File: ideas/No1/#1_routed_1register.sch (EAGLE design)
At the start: 20 parts, among them P1-O8RIGHT TD620831A, P1-P8LEFT TD620831A, U1 SN74HC595N, U2 SN74HC595N, U3 SN74HC595N

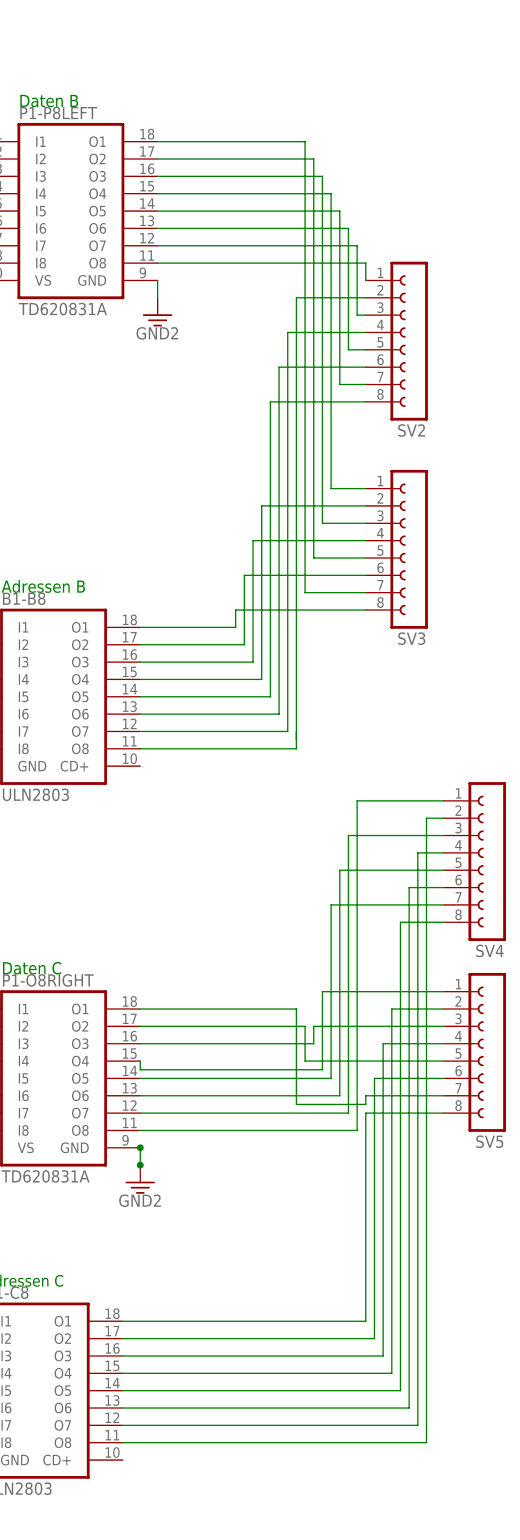
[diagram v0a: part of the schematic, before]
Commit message: 1_route_1register.sch updated
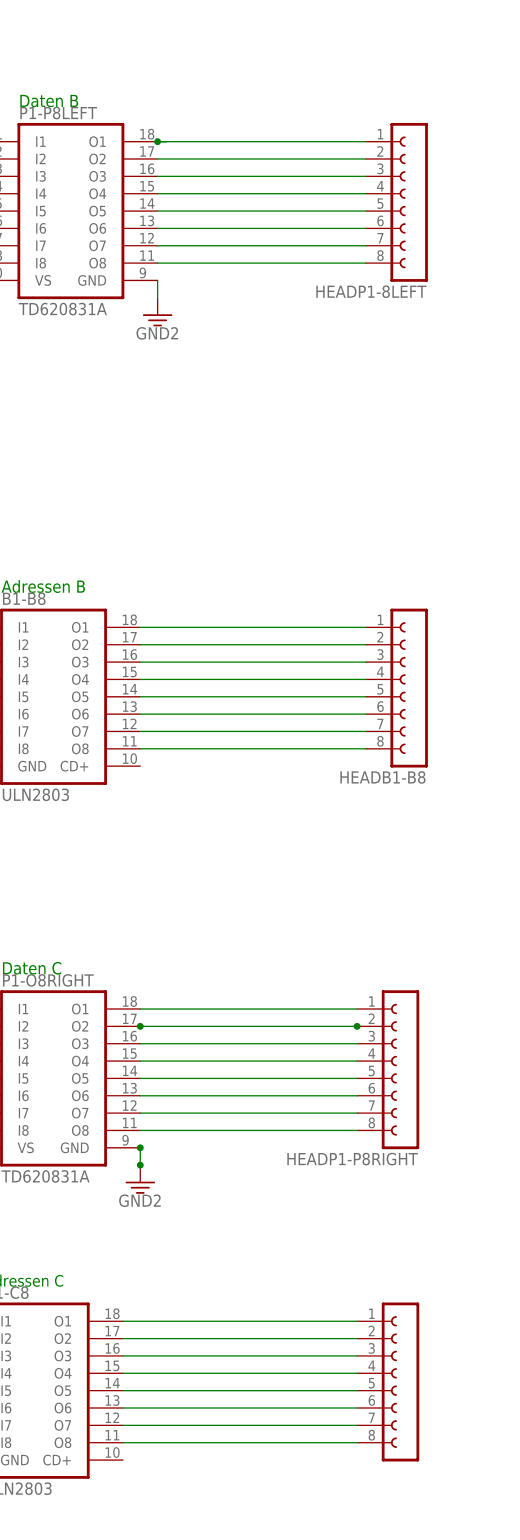
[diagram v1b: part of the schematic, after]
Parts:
- removed SV2, SV3, SV4, SV5: (no value), con-lsta:FE08-1
- added HEADB1-B8, HEADC1-C8, HEADP1-8LEFT, HEADP1-P8RIGHT: (no value), con-lsta:FE08-1
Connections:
- removed net N$60: C1-C8.O8, SV4.2
- new net N$20: HEADP1-8LEFT.1, P1-P8LEFT.O1
- net N$10: now also HEADP1-8LEFT.3, P1-P8LEFT.O3; no longer P1-P8LEFT.O7, SV2.3
- net N$11: now also HEADP1-8LEFT.4, P1-P8LEFT.O4; no longer P1-P8LEFT.O6, SV2.5
- net N$12: now also HEADP1-8LEFT.5, P1-P8LEFT.O5; no longer B1-B8.O4, SV3.2
- net N$13: now also HEADP1-8LEFT.6, P1-P8LEFT.O6; no longer P1-P8LEFT.O5, SV2.7
- net N$14: now also HEADP1-8LEFT.7, P1-P8LEFT.O7; no longer P1-P8LEFT.O4, SV3.1
- net N$15: now also HEADP1-8LEFT.8, P1-P8LEFT.O8; no longer P1-P8LEFT.O3, SV3.3
- net N$16: now also B1-B8.O1, HEADB1-B8.1; no longer P1-P8LEFT.O2, SV3.5
- net N$17: now also B1-B8.O2, HEADB1-B8.2; no longer P1-P8LEFT.O1, SV3.7
- net N$18: now also B1-B8.O3, HEADB1-B8.3; no longer B1-B8.O8, SV2.2
- net N$19: now also B1-B8.O4, HEADB1-B8.4; no longer B1-B8.O7, SV2.4
- net N$21: now also B1-B8.O5, HEADB1-B8.5; no longer B1-B8.O6, SV2.6
- net N$22: now also B1-B8.O6, HEADB1-B8.6; no longer B1-B8.O5, SV2.8
- net N$23: now also B1-B8.O7, HEADB1-B8.7; no longer B1-B8.O3, SV3.4
- net N$24: now also B1-B8.O8, HEADB1-B8.8; no longer B1-B8.O2, SV3.6
- net N$26: now also HEADP1-P8RIGHT.1, P1-O8RIGHT.O1; no longer B1-B8.O1, SV3.8
- net N$28: now also HEADP1-P8RIGHT.3, P1-O8RIGHT.O3; no longer P1-O8RIGHT.O7, SV4.3
- net N$30: now also HEADP1-P8RIGHT.2, P1-O8RIGHT.O2; no longer P1-O8RIGHT.O8, SV4.1
- net N$33: now also HEADP1-P8RIGHT.5, P1-O8RIGHT.O5; no longer C1-C8.O2, SV5.6
- net N$35: now also HEADP1-P8RIGHT.6, P1-O8RIGHT.O6; no longer P1-O8RIGHT.O5, SV4.7
- net N$39: now also HEADP1-P8RIGHT.4; no longer SV5.1
- net N$40: now also HEADP1-P8RIGHT.7, P1-O8RIGHT.O7; no longer P1-O8RIGHT.O3, SV5.3
- net N$49: now also HEADP1-P8RIGHT.8, P1-O8RIGHT.O8; no longer P1-O8RIGHT.O6, SV4.5
- net N$50: now also C1-C8.O1, HEADC1-C8.1; no longer P1-O8RIGHT.O2, SV5.5
- net N$51: now also C1-C8.O2, HEADC1-C8.2; no longer P1-O8RIGHT.O1, SV5.7
- net N$52: now also C1-C8.O3, HEADC1-C8.3; no longer C1-C8.O1, SV5.8
- net N$53: now also C1-C8.O4, HEADC1-C8.4; no longer C1-C8.O3, SV5.4
- net N$54: now also C1-C8.O5, HEADC1-C8.5; no longer C1-C8.O4, SV5.2
- net N$57: now also C1-C8.O6, HEADC1-C8.6; no longer C1-C8.O5, SV4.8
- net N$58: now also C1-C8.O7, HEADC1-C8.7; no longer C1-C8.O6, SV4.6
- net N$59: now also C1-C8.O8, HEADC1-C8.8; no longer C1-C8.O7, SV4.4
- net N$9: now also HEADP1-8LEFT.2, P1-P8LEFT.O2; no longer P1-P8LEFT.O8, SV2.1
